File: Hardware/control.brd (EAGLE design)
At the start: 100 x 80 mm, 11 parts, among them IC1 317T

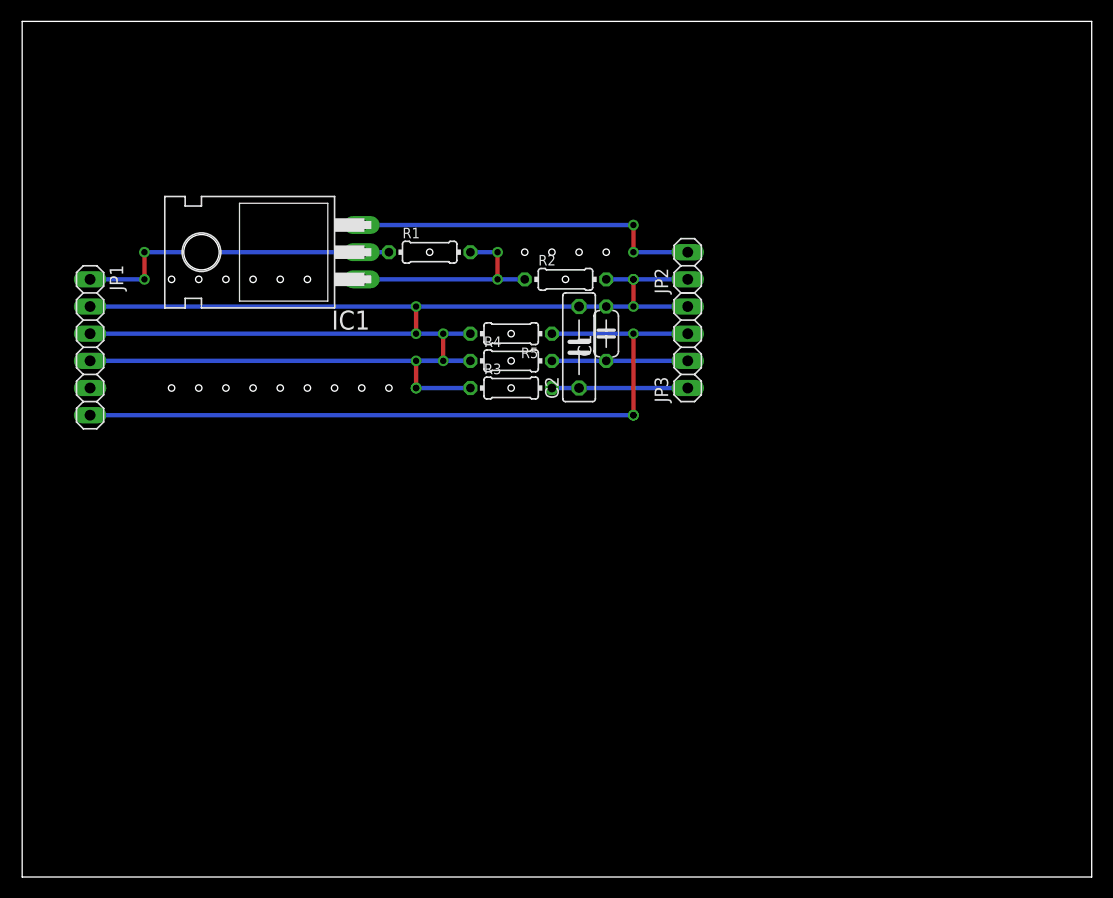
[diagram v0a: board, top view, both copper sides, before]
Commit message: Added some better schematics
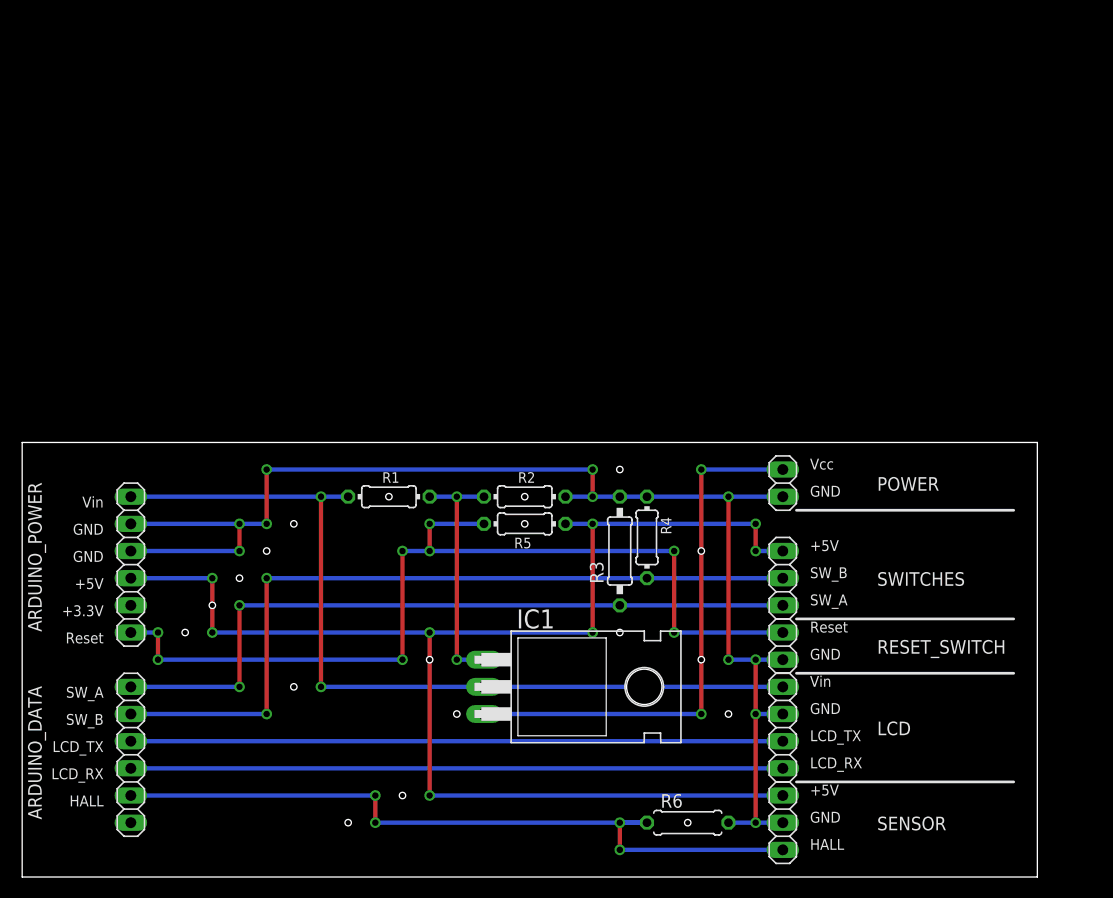
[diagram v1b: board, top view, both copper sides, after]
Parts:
- removed C1: 100uF, Rodentometer:C050-024X044
- removed C2: 100uF, Rodentometer:C075-032X103
- removed JP1: (no value), Rodentometer:1X06
- removed JP2: (no value), Rodentometer:1X02
- removed JP3: (no value), Rodentometer:1X04
- added ARDUINO_DATA, ARDUINO_POWER: (no value), Rodentometer:1X06
- added LCD: (no value), Rodentometer:1X04
- added POWER, RESET_SWITCH: (no value), Rodentometer:1X02
- added R6: 10k, Rodentometer:0207/7
- added SENSOR, SWITCHES: (no value), Rodentometer:1X03
- R3: device Rodentometer:0204/7 -> Rodentometer:0207/10
- moved IC1 51.6 mm to (53.3, 17.8), turned to 270 degrees
- moved R1 23.2 mm to (34.3, 35.6)
- moved R4 20.8 mm to (58.4, 31.8), turned to 90 degrees
- moved R2 20.7 mm to (47.0, 35.6)
- moved R3 18.3 mm to (55.9, 30.5), turned to 90 degrees
- moved R5 17.8 mm to (47.0, 33.0), turned to 0 degrees
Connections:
- removed net N$1: IC1.2, JP1.1, R1.1
- removed net N$2: IC1.3, JP2.2
- removed net N$3: C2.1, JP3.1, R3.2
- removed net N$4: C1.1, JP3.2, R4.2
- removed net N$6: JP1.6, JP3.3, R5.1
- new net HALL: ARDUINO_DATA.5, R6.1, SENSOR.3
- new net LCD_RX: ARDUINO_DATA.4, LCD.4
- new net LCD_TX: ARDUINO_DATA.3, LCD.3
- new net RESET: ARDUINO_POWER.6, R5.1, RESET_SWITCH.1
- new net SW_A: ARDUINO_DATA.1, R3.1, SWITCHES.1
- new net SW_B: ARDUINO_DATA.2, R4.1, SWITCHES.2
- new net VCC: IC1.3, POWER.2
- new net VIN: ARDUINO_POWER.1, IC1.2, LCD.1, R1.1
- net +5V: now also ARDUINO_POWER.4, SENSOR.1, SWITCHES.3; no longer JP1.4, R3.1, R4.1
- net GND: now also ARDUINO_POWER.2, ARDUINO_POWER.3, LCD.2, POWER.1, R3.2, R4.2, R6.2, RESET_SWITCH.2, SENSOR.2; no longer C1.2, C2.2, JP1.2, JP1.3, JP2.1, JP3.4
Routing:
- net RESET: track 0.00 -> 88.9 mm, vias 0 -> 8
- net VIN: track 0.00 -> 81.3 mm, vias 0 -> 2
- net +5V: track 53.3 -> 129.5 mm, vias 4 -> 8
- net SW_B: track 0.00 -> 73.7 mm, vias 0 -> 2
- net HALL: track 0.00 -> 71.1 mm, vias 0 -> 4
- net N$6: track 71.1 -> 0.00 mm, vias 2 -> 0
- net SW_A: track 0.00 -> 68.6 mm, vias 0 -> 2
- net LCD_TX: track 0.00 -> 61.0 mm
- net LCD_RX: track 0.00 -> 61.0 mm
- net VCC: track 0.00 -> 50.8 mm, vias 0 -> 2
- net N$2: track 33.0 -> 0.00 mm, vias 2 -> 0
- net N$1: track 30.5 -> 0.00 mm, vias 2 -> 0
- net GND: track 101.6 -> 127.0 mm, vias 5 -> 11
- net N$4: track 12.7 -> 0.00 mm
- net N$3: track 12.7 -> 0.00 mm
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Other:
- board size 100 x 80 mm -> 94.9 x 40.6 mm
- board text added: "+3.3V"
- board text added: "+5V"
- board text added: "GND"
- board text added: "HALL"
- board text added: "LCD_RX"
- board text added: "LCD_TX"
- board text added: "Reset"
- board text added: "SW_A"
- board text added: "SW_B"
- board text added: "Vcc"
- board text added: "Vin"
